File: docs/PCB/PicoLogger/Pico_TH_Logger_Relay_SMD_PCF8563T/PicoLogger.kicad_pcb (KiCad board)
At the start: 2 copper layers, 100.5 x 83 mm, 63 parts, among them J1 Sensor, J2 LCD 16x2, J3 Additional connector, J4 K4_Output, J5 K3_Output, J6 K2_Output, J7 K1_Output, J8 SPI, K1 G5Q-1, K2 G5Q-1, K3 G5Q-1, K4 G5Q-1, Q1 MMBT3904, Q2 MMBT3904, Q3 MMBT3904, Q4 MMBT3904, SW1 SW_Push, SW2 SW_Push, U1 LTV-817S, U2 LTV-817S, U3 LTV-817S, U4 LTV-817S, U5 PCF8563T, Y1 Crystal

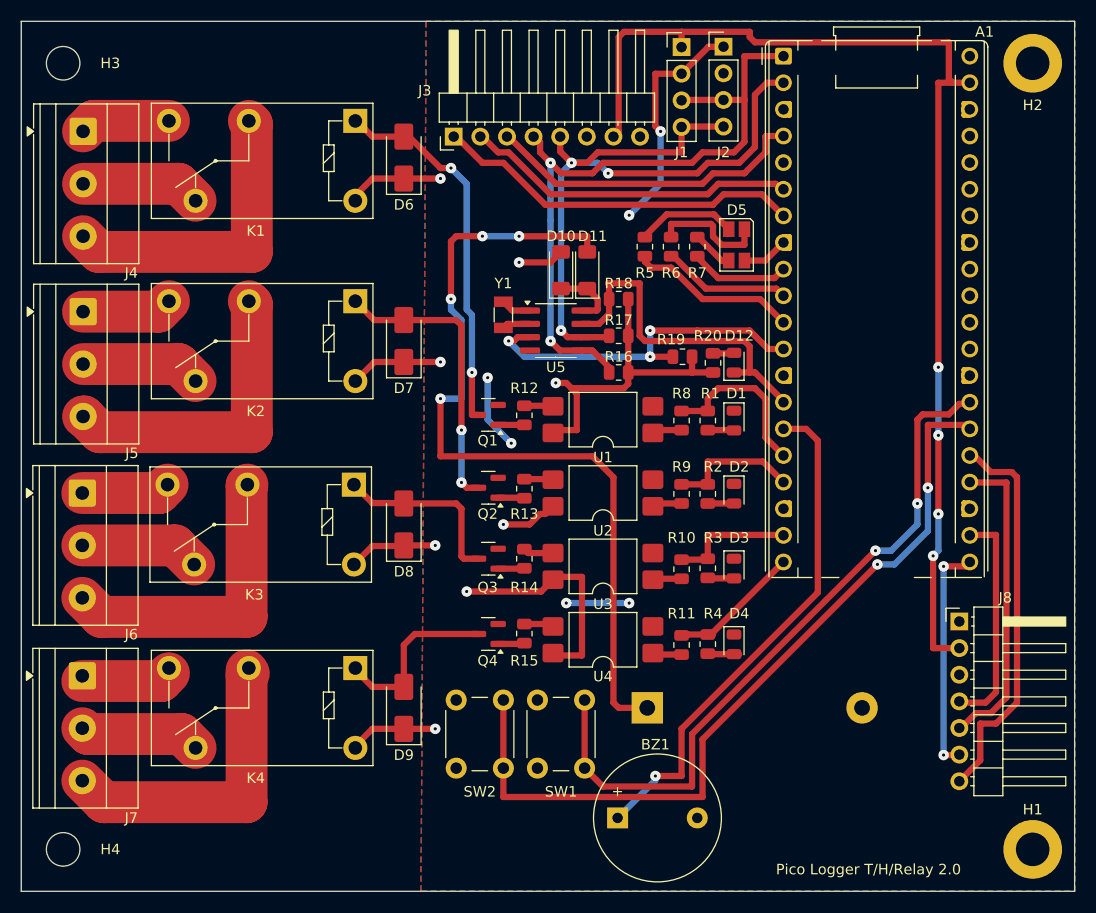
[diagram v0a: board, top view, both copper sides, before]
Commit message: Updated docs.
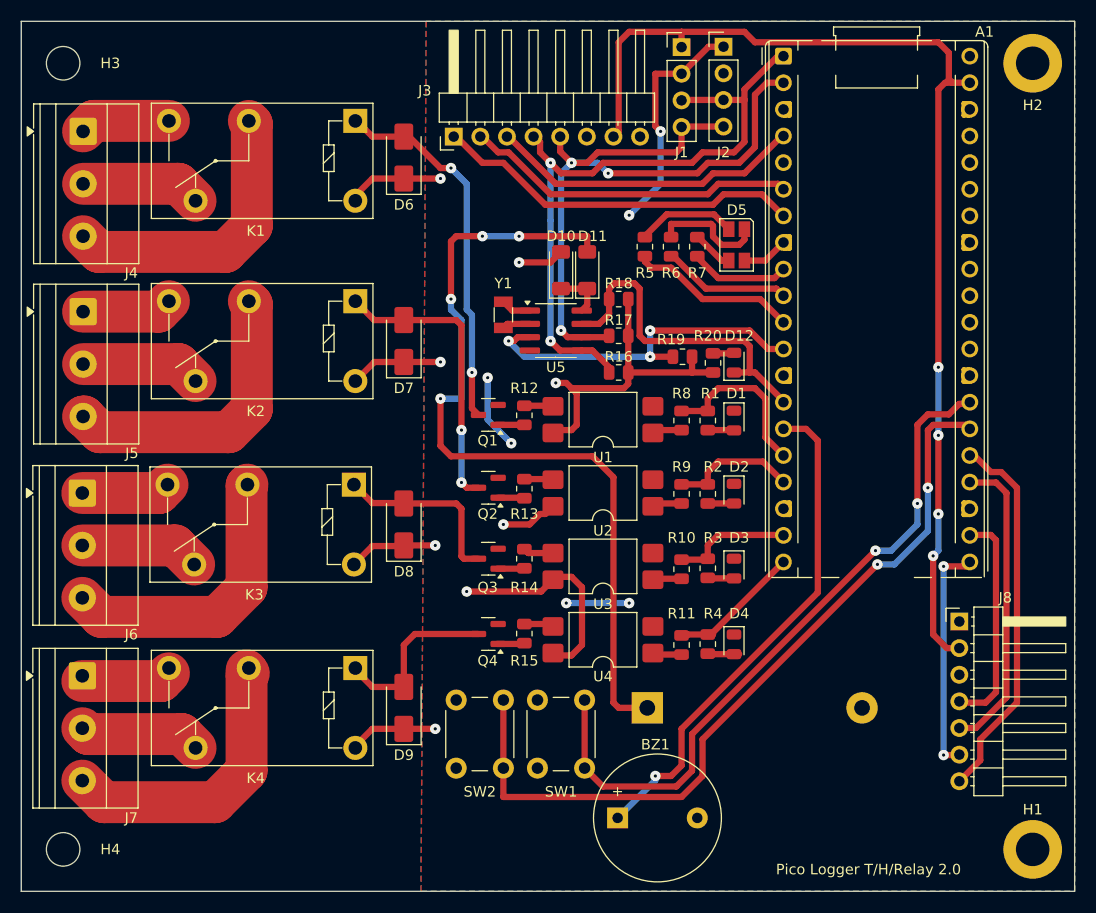
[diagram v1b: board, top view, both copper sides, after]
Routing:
- net +3.3V: track 106.7 -> 104.4 mm
- net SDA: track 65.4 -> 63.5 mm
- net K4_Pin2: track 29.4 -> 27.7 mm
- net Net-(D10-K): track 6.48 -> 4.81 mm
- net K3_Pin2: track 29.1 -> 27.4 mm
- net SPI TX: track 38.0 -> 36.6 mm
- net K1_Pin5: track 97.8 -> 96.4 mm
- net K1_Pin2: track 29.3 -> 27.9 mm
- net GPIO20: track 77.8 -> 76.3 mm
- net K2_Pin2: track 29.3 -> 28.1 mm
- net GPIO21: track 67.9 -> 66.8 mm
- net GPIO2: track 31.2 -> 30.3 mm
- net GPIO10: track 33.2 -> 32.5 mm
- net +BATT: track 79.9 -> 79.3 mm
- net GPIO11: track 49.1 -> 48.5 mm
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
